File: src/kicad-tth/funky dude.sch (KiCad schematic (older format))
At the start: 30 parts, among them P1 CONN_2, P2 CONN_2, P3 CONN_2, U1 OP284

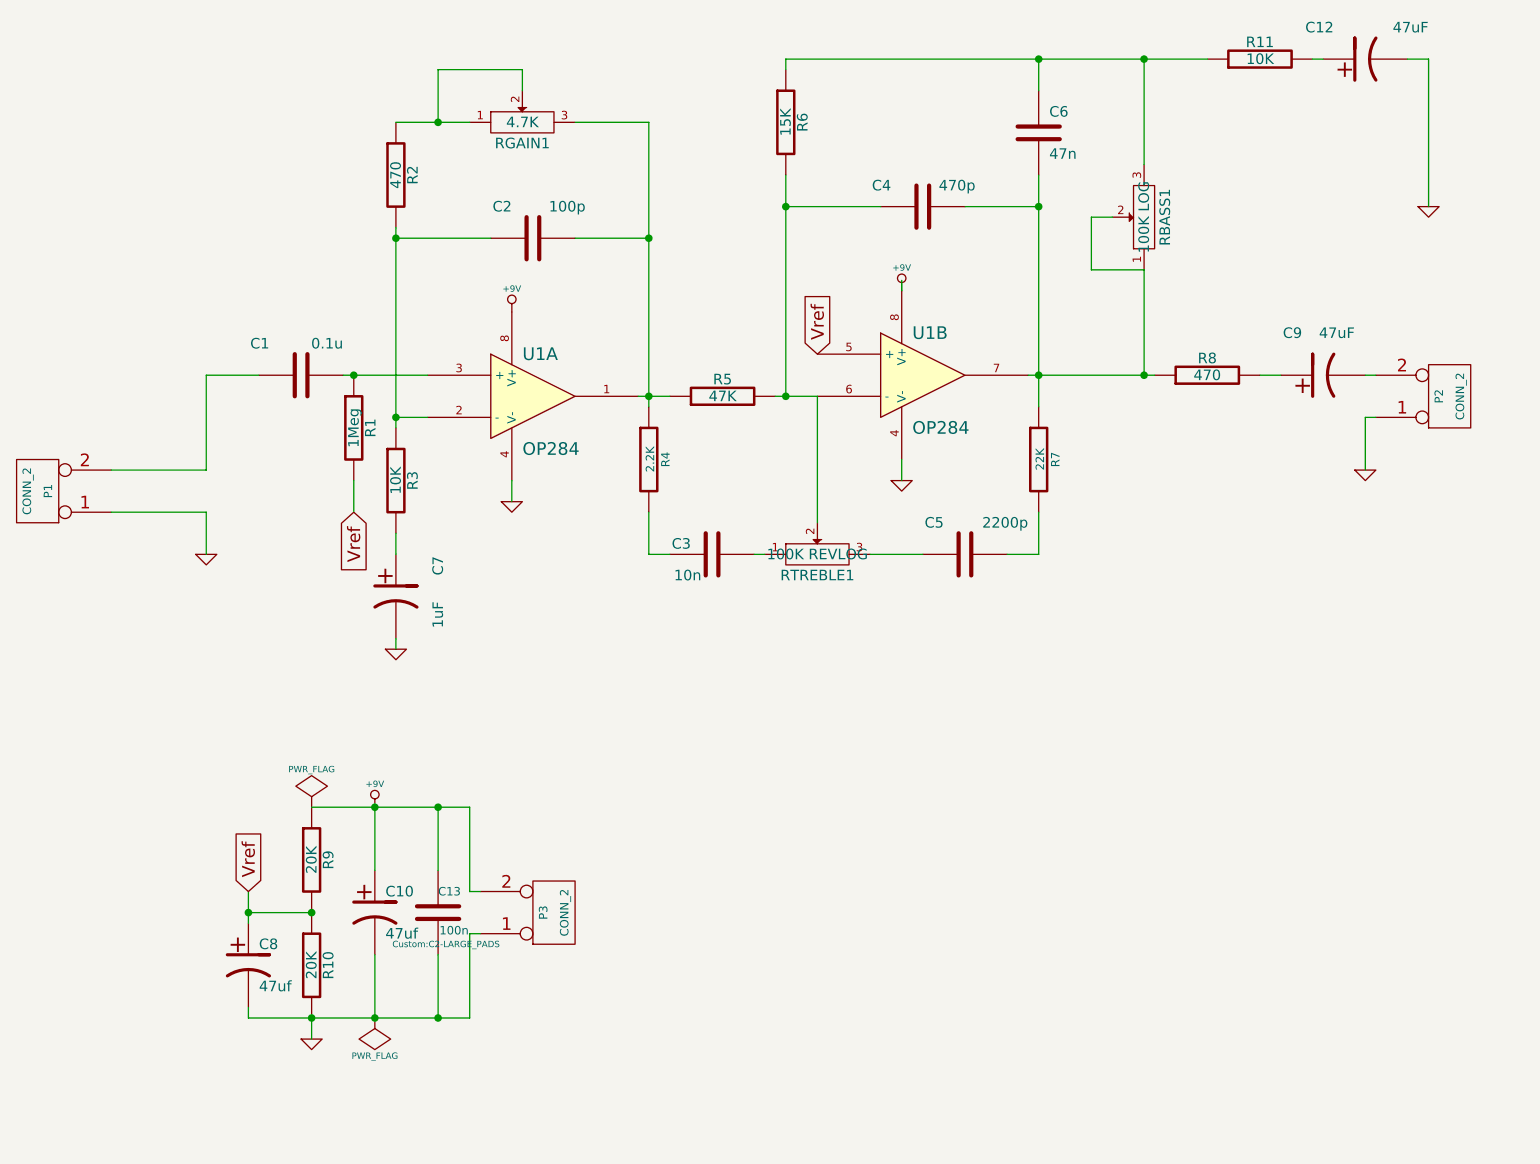
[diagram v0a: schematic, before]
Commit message: 2014-10-23.2 - PCB is routed
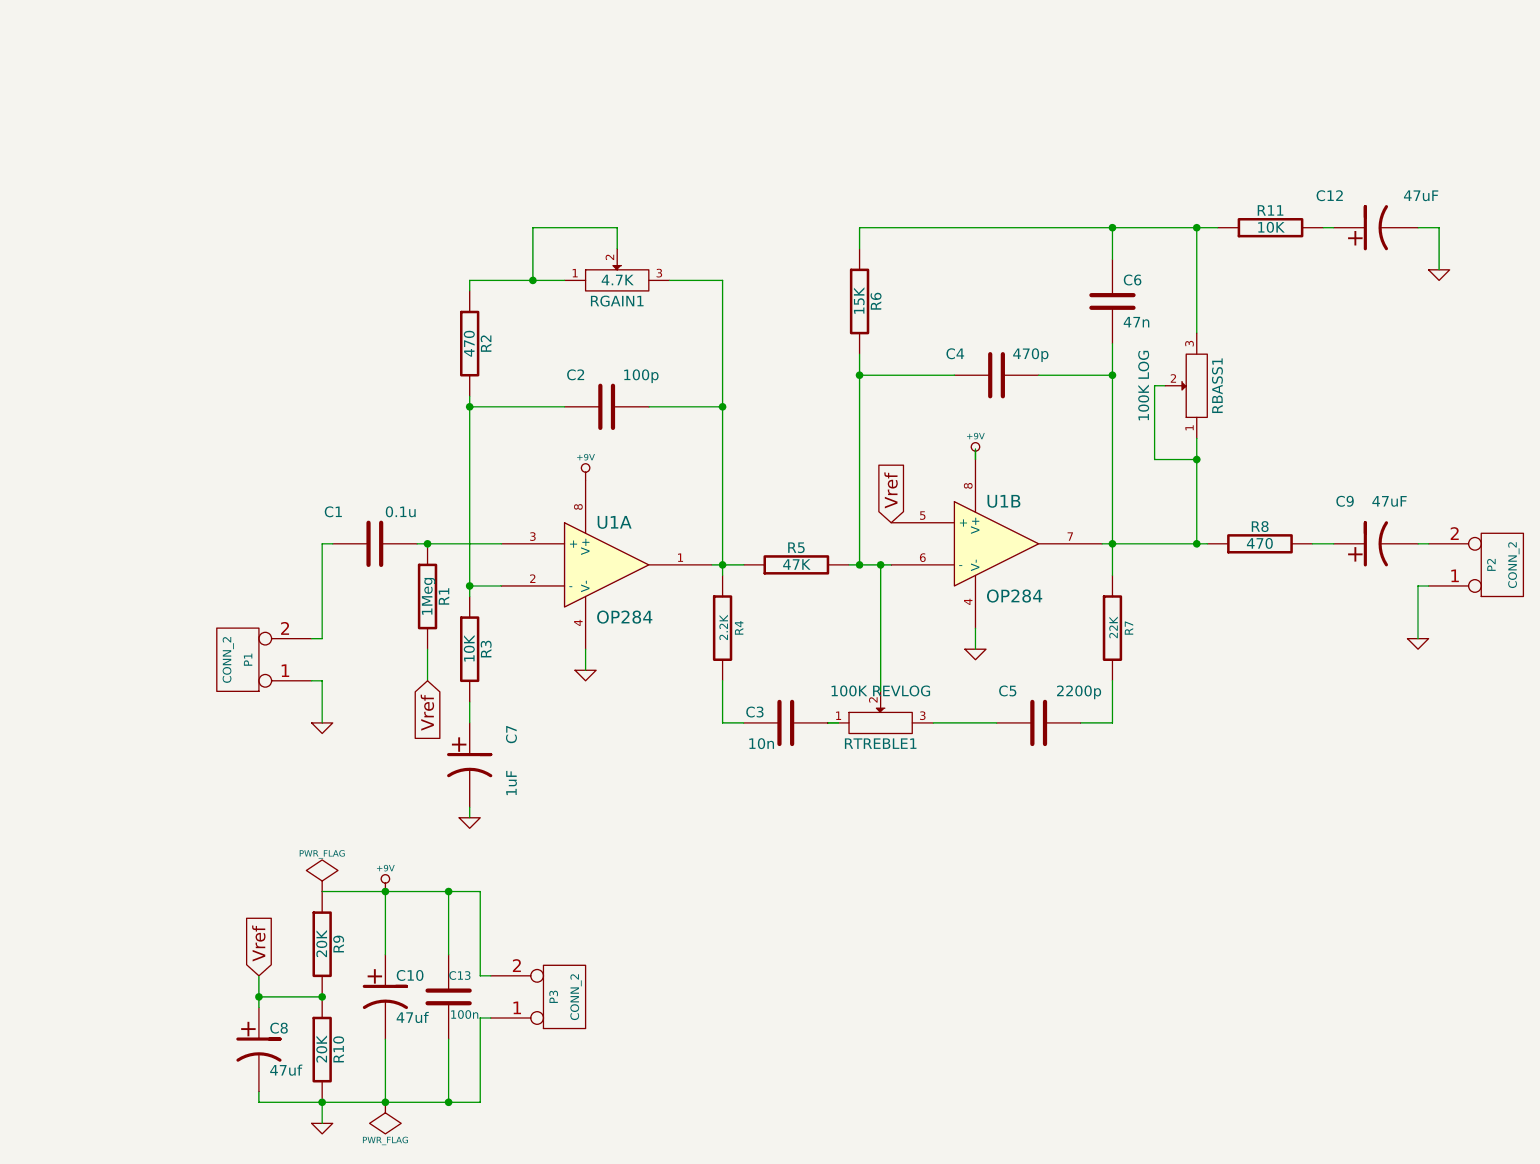
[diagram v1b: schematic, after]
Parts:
- C13: footprint Custom:C2-LARGE_PADS -> (none)
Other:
- moved on the sheet: C1, C10, C12, C13, C2, C3, C4, C5, C6, C7, C8, C9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
